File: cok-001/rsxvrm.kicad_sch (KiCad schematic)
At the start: 12 parts, among them U6201 NCP5318FTR2G, U6202 iP2003APbF, U6203 iP2003APbF, U6204 TC7SG08FU

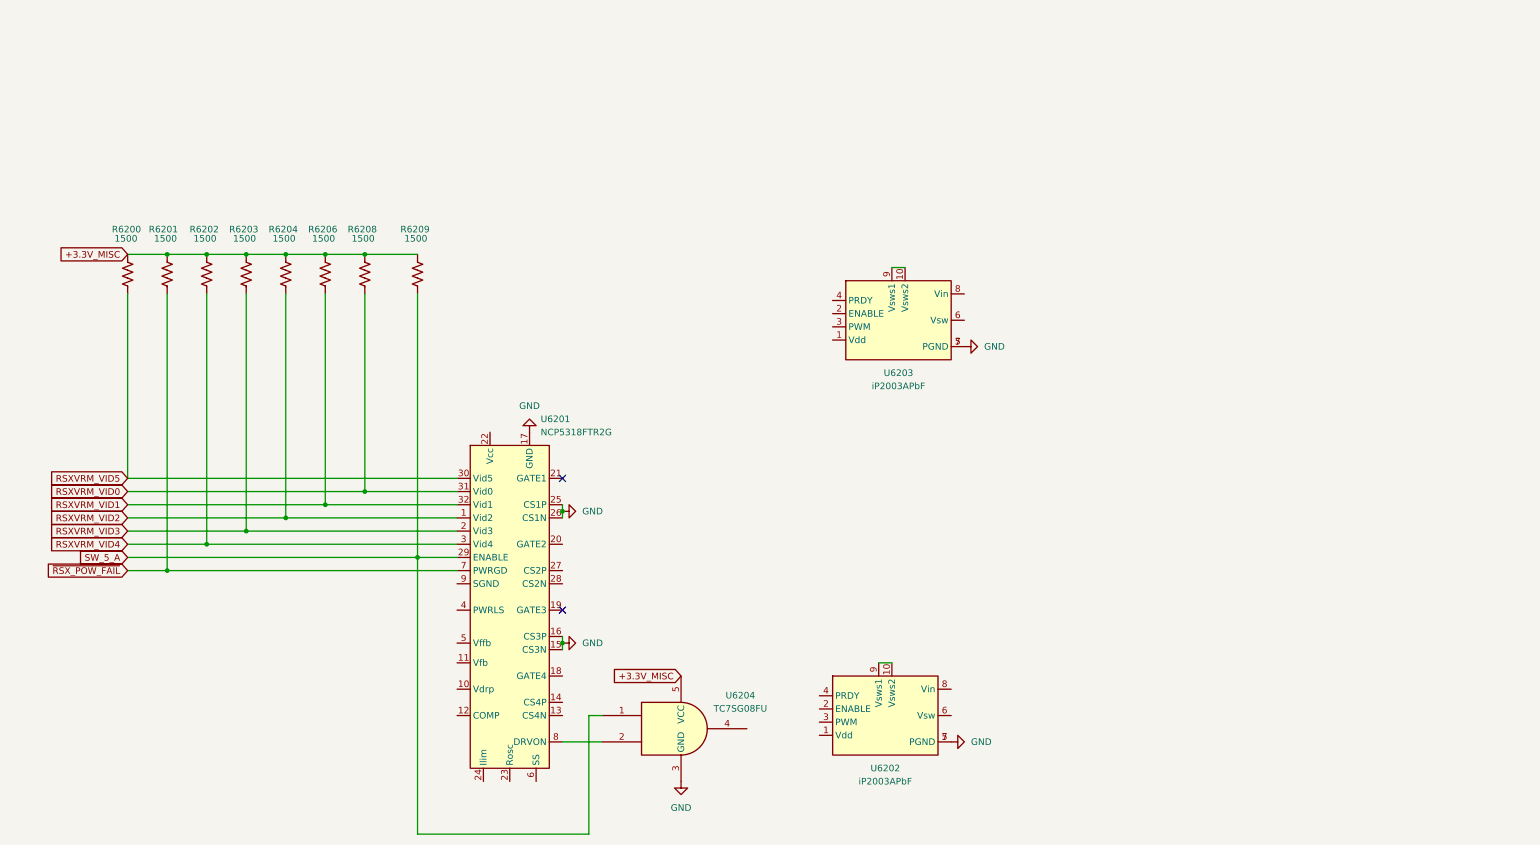
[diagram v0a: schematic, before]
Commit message: rsx
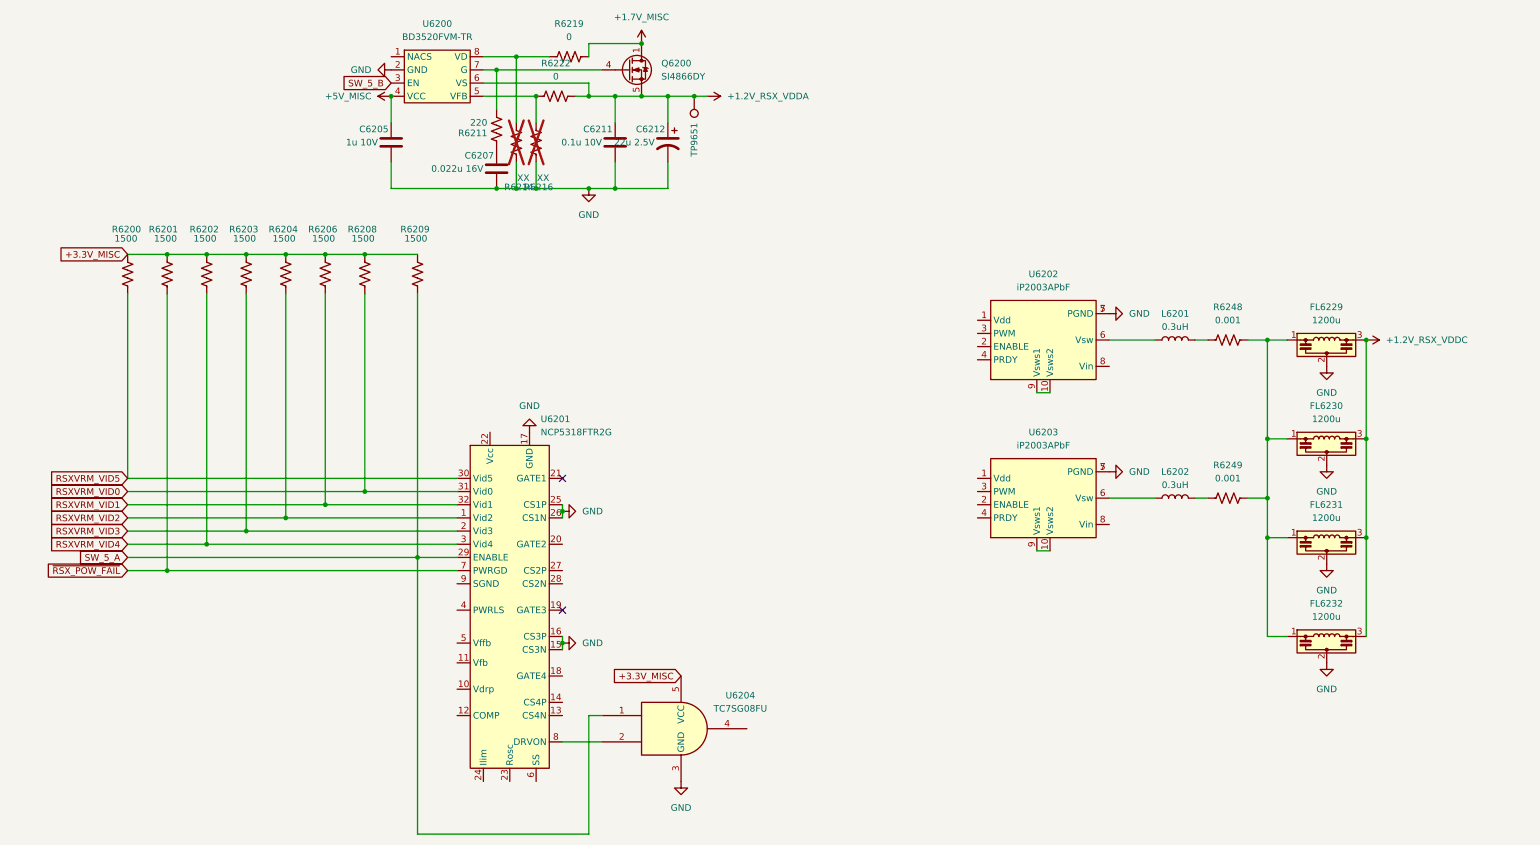
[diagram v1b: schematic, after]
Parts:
- added C6205: 1u 10V, Capacitor_SMD:C_0402_1005Metric, symbol Device:C
- added C6207: 0.022u 16V, Capacitor_SMD:C_0402_1005Metric, symbol Device:C
- added C6211: 0.1u 10V, Capacitor_SMD:C_0402_1005Metric, symbol Device:C
- added C6212: 22u 2.5V, Capacitor_SMD:C_0402_1005Metric, symbol Device:C_Polarized_US
- added FL6229, FL6230, FL6231, FL6232: 1200u, PS3:Proadlizer, symbol Device:Filter_EMI_CLC
- added L6201, L6202: 0.3uH, Inductor_SMD:L_Bourns_SRR1208_12.7x12.7mm, symbol Device:L
- added Q6200: SI4866DY, Package_SO:SSOP-8_3.9x5.05mm_P1.27mm, symbol Transistor_FET:IRF7607PBF
- added R6211: 220, Resistor_SMD:R_0402_1005Metric, symbol Device:R_US
- added R6214, R6216: XX, Resistor_SMD:R_0402_1005Metric, symbol Device:R_US
- added R6219, R6222: 0, Resistor_SMD:R_0402_1005Metric, symbol Device:R_US
- added R6248, R6249: 0.001, Resistor_SMD:R_2512_6332Metric, symbol Device:R_US
- added TP9651: TestPoint, TestPoint:TestPoint_Pad_D1.5mm, symbol Connector:TestPoint
- added U6200: BD3520FVM-TR, Package_SO:MSOP-8_3x3mm_P0.65mm, symbol PS3:BD35xxFVM-TR
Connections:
- net GND: now also C6205.2, C6207.2, C6211.2, C6212.2, FL6229.2, FL6230.2, FL6231.2, FL6232.2, R6214.1, R6216.1, U6200.2 (GND)
- net at U6203.6 (Vsw): now also L6202.1
- net at U6202.6 (Vsw): now also L6201.1
- new net: FL6229.1, FL6230.1, FL6231.1, FL6232.1, R6248.2, R6249.2
- new net: C6207.1, R6211.1
- new net: Q6200.4 (G), R6211.2, U6200.7 (G)
- new net: R6216.2, R6222.1, U6200.5 (VFB)
- new net: R6214.2, R6219.1, U6200.8 (VD)
- new net: L6202.2, R6249.1
- new net: L6201.2, R6248.1
- new net +1.2V_RSX_VDDA: C6211.1, C6212.1, Q6200.5 (D), Q6200.6 (D), Q6200.7 (D), Q6200.8 (D), R6222.2, TP9651.1, U6200.6 (VS)
- new net +1.2V_RSX_VDDC: FL6229.3, FL6230.3, FL6231.3, FL6232.3
- new net +1.7V_MISC: Q6200.1 (S), Q6200.2 (S), Q6200.3 (S), R6219.2
- new net +5V_MISC: C6205.1, U6200.4 (VCC)
- new net SW_5_B: U6200.3 (EN)
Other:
- moved on the sheet: U6202, U6203

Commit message: msop
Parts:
- U6200: footprint Package_SO:MSOP-8_3x3mm_P0.65mm -> PS3:MSOP-8_2.9x4mm_P0.65mm
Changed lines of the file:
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@@
 			)
 		)
-		(property "Footprint" "Package_SO:MSOP-8_3x3mm_P0.65mm"
+		(property "Footprint" "PS3:MSOP-8_2.9x4mm_P0.65mm"
 			(at 78.74 25.4 0)
 			(effects

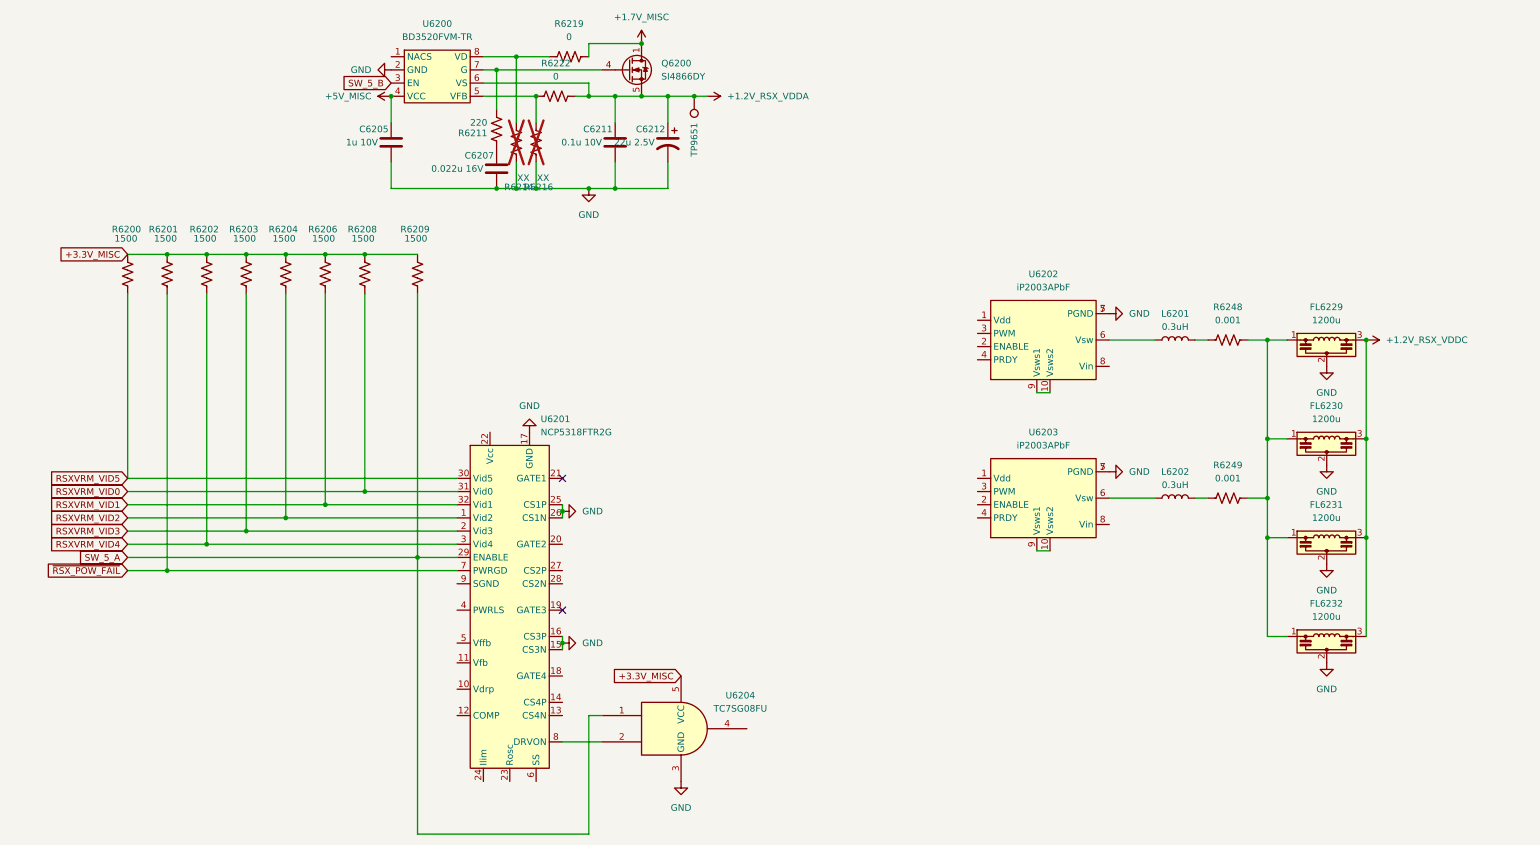
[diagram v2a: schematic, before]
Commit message: pid in
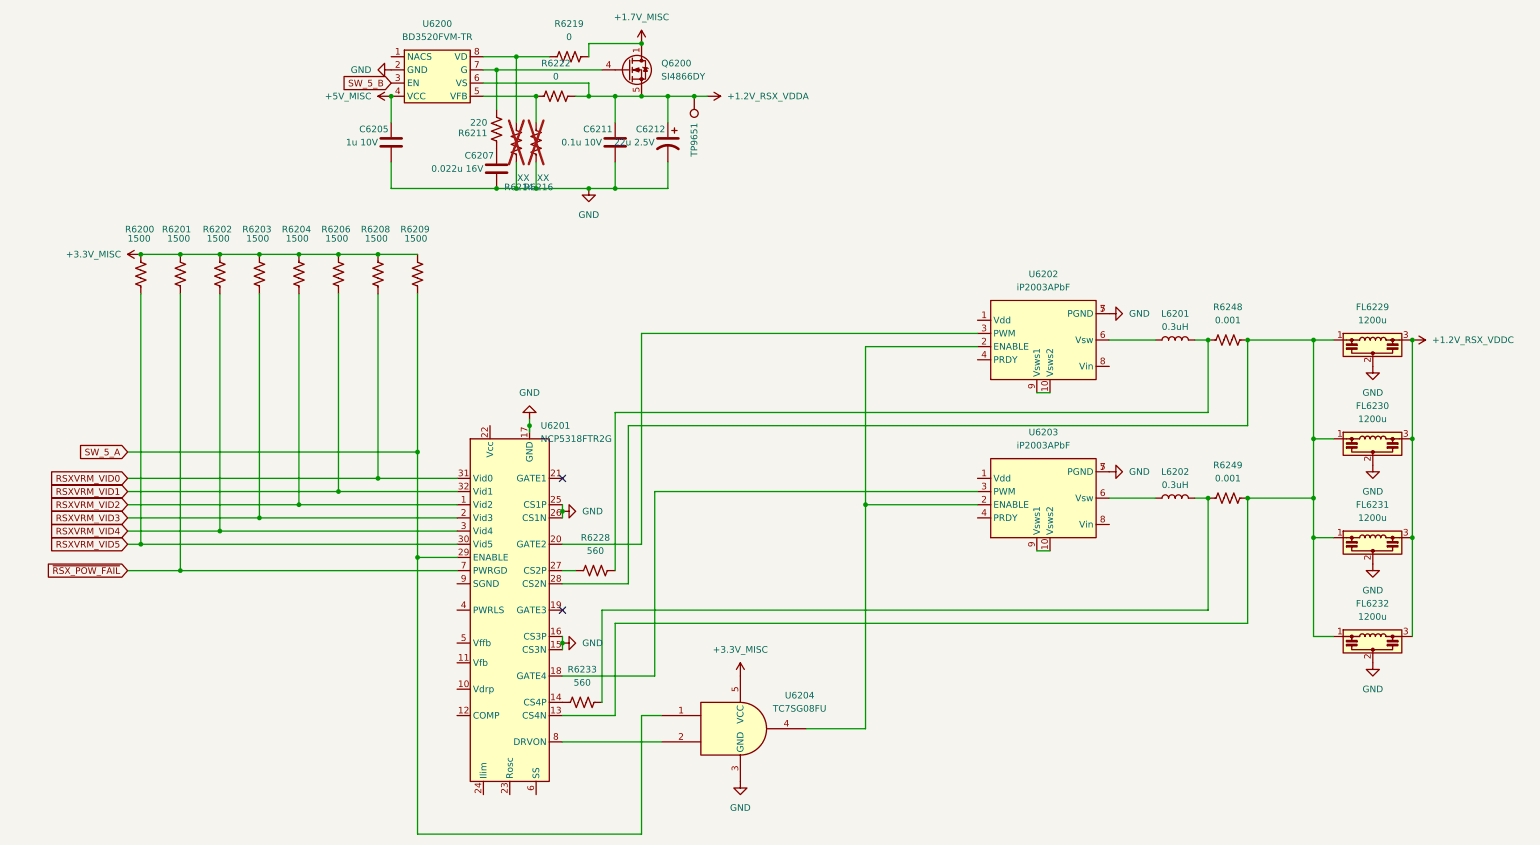
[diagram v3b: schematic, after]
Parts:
- added R6228, R6233: 560, Resistor_SMD:R_0402_1005Metric, symbol Device:R_US
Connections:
- net at U6203.2 (ENABLE): now also U6202.2 (ENABLE), U6204.4
- net at U6203.3 (PWM): now also U6201.18 (GATE4)
- net at FL6229.1, FL6230.1, FL6231.1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: now also U6201.13 (CS4N), U6201.28 (CS2N)
- net at L6202.2, R6249.1: now also R6233.2
- net at L6201.2, R6248.1: now also R6228.2
- net at U6201.14 (CS4P): now also R6233.1
- net at U6201.20 (GATE2): now also U6202.3 (PWM)
- net at U6201.27 (CS2P): now also R6228.1
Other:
- moved on the sheet: FL6229, FL6230, FL6231, FL6232, R6200, R6201, R6202, R6203, R6204, R6206, R6208, U6201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
